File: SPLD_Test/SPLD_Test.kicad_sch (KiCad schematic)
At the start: 34 parts, among them J1 SPI OLED 1.3in, J2 USB_C_Receptacle_PowerOnly_6P, J3 Conn_02x09_Top_Bottom, J4 SWD, J5 Conn_02x09_Top_Bottom, J6 Conn_02x09_Top_Bottom, SW1 SW_MEC_5E, SW2 SW_MEC_5E, SW3 SW_MEC_5E, SW4 SW_MEC_5E, U1 STM32F030K6Tx, U2 EA8105, U3 CA56-12CGKWA, U4 ATF1502ASV-xAx44

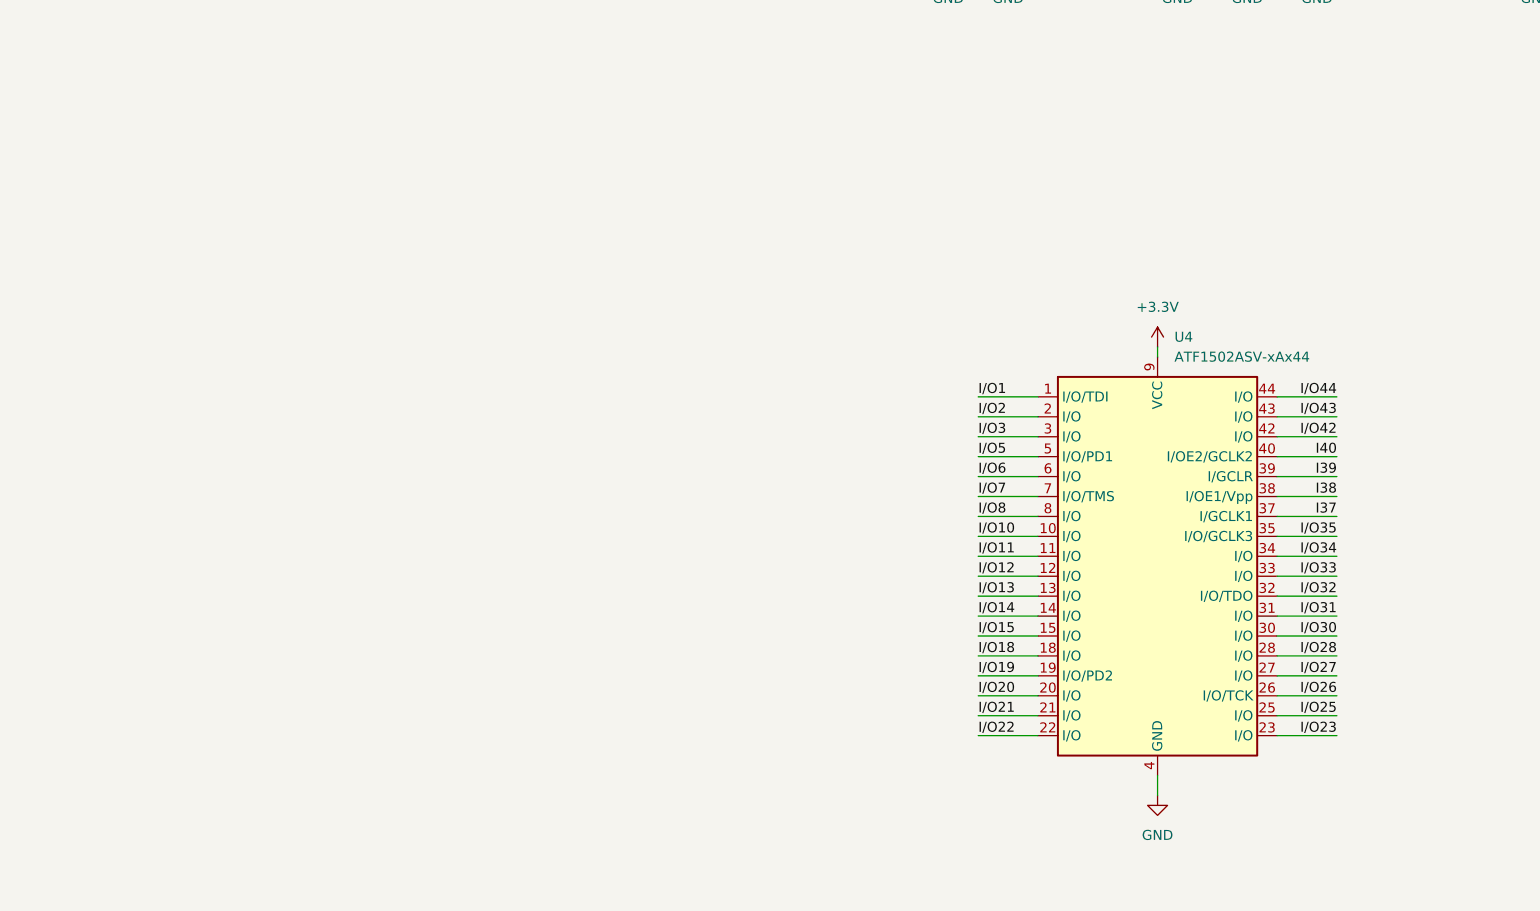
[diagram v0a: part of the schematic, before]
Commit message: progress: CPLD Big Change
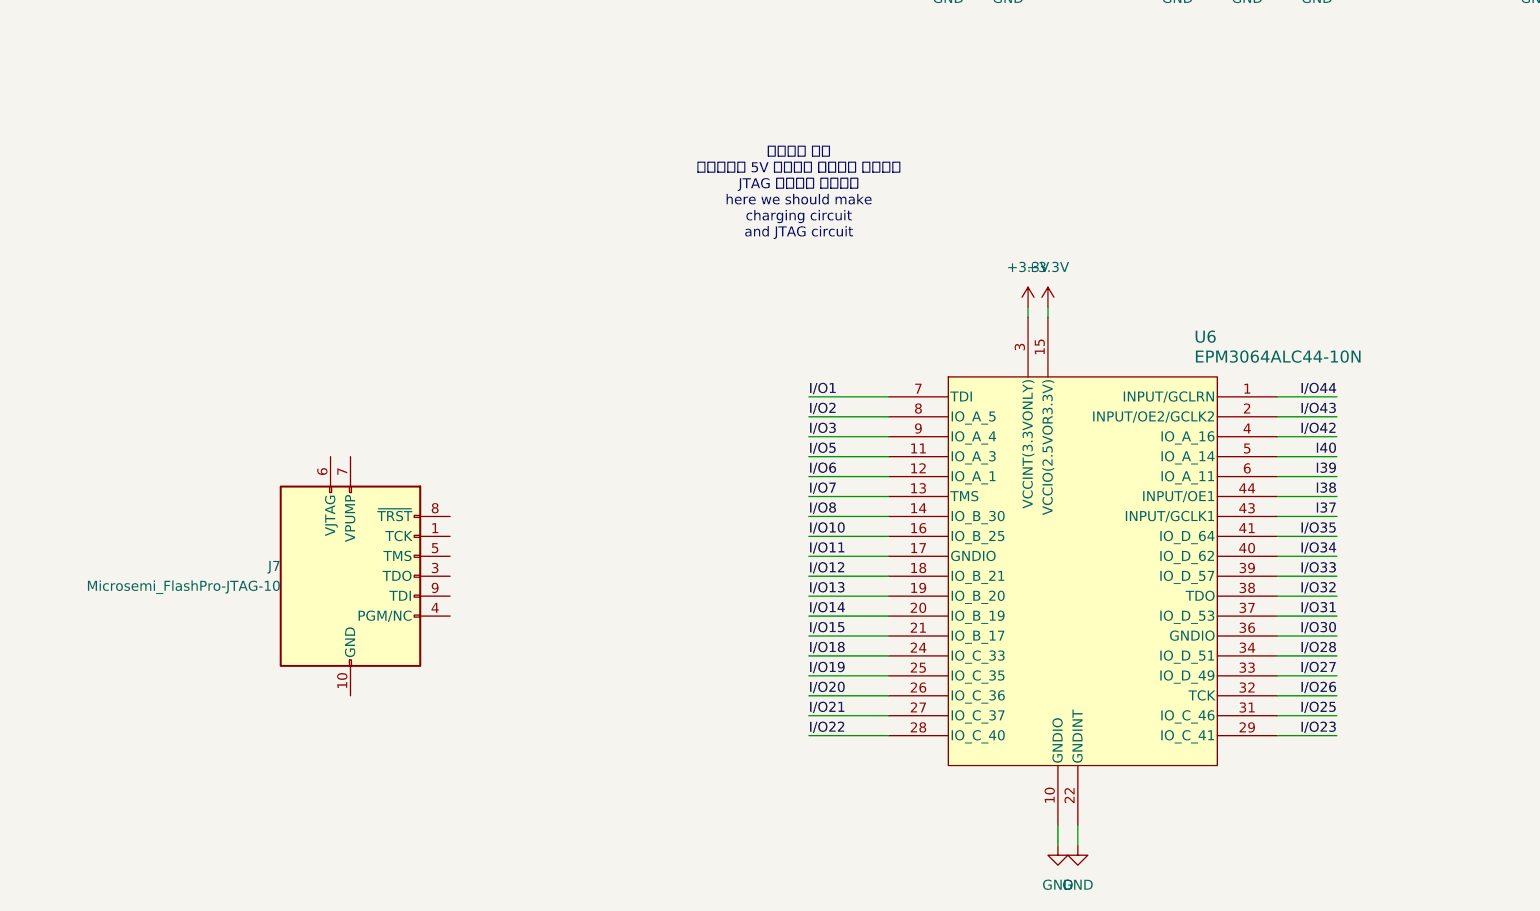
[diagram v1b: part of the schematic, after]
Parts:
- removed U4: ATF1502ASV-xAx44, Package_LCC:PLCC-44_THT-Socket, symbol CPLD_Microchip:ATF1502ASV-xAx44
- added J7: Microsemi_FlashPro-JTAG-10, Connector_IDC:IDC-Header_2x05_P2.54mm_Vertical, symbol Connector:Microsemi_FlashPro-JTAG-10
- added U6: EPM3064ALC44-10N, Package_LCC:PLCC-44_THT-Socket, symbol GH_LIBRARIES:EPM3064ALC44-10N
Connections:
- net +3.3V: now also U6.15 (VCCIO(2.5VOR3.3V)), U6.23 (VCCINT(3.3VONLY)), U6.3 (VCCINT(3.3VONLY)), U6.35 (VCCIO(2.5VOR3.3V))
- net GND: now also U6.10 (GNDIO), U6.22 (GNDINT), U6.30 (GNDIO), U6.42 (GNDINT)
- net I37: now also U6.43 (INPUT/GCLK1)
- net I38: now also U6.44 (INPUT/OE1)
- net I39: now also U6.6 (IO_A_11)
- net I40: now also U6.5 (IO_A_14)
- net I/O1: now also U6.7 (TDI)
- net I/O10: now also U6.16 (IO_B_25)
- net I/O11: now also U6.17 (GNDIO)
- net I/O12: now also U6.18 (IO_B_21)
- net I/O13: now also U6.19 (IO_B_20)
- net I/O14: now also U6.20 (IO_B_19)
- net I/O15: now also U6.21 (IO_B_17)
- net I/O18: now also U6.24 (IO_C_33)
- net I/O19: now also U6.25 (IO_C_35)
- net I/O2: now also U6.8 (IO_A_5)
- net I/O20: now also U6.26 (IO_C_36)
- net I/O21: now also U6.27 (IO_C_37)
- net I/O22: now also U6.28 (IO_C_40)
- net I/O23: now also U6.29 (IO_C_41)
- net I/O25: now also U6.31 (IO_C_46)
- net I/O26: now also U6.32 (TCK)
- net I/O27: now also U6.33 (IO_D_49)
- net I/O28: now also U6.34 (IO_D_51)
- net I/O3: now also U6.9 (IO_A_4)
- net I/O30: now also U6.36 (GNDIO)
- net I/O31: now also U6.37 (IO_D_53)
- net I/O32: now also U6.38 (TDO)
- net I/O33: now also U6.39 (IO_D_57)
- net I/O34: now also U6.40 (IO_D_62)
- net I/O35: now also U6.41 (IO_D_64)
- net I/O42: now also U6.4 (IO_A_16)
- net I/O43: now also U6.2 (INPUT/OE2/GCLK2)
- net I/O44: now also U6.1 (INPUT/GCLRN)
- net I/O5: now also U6.11 (IO_A_3)
- net I/O6: now also U6.12 (IO_A_1)
- net I/O7: now also U6.13 (TMS)
- net I/O8: now also U6.14 (IO_B_30)
- new net: J7.10 (GND), J7.2 (GND)
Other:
- note added: "여기다가 그거 충전회로와 5V 승압회로 만들어서 적용하기 JTAG 만들어서 적용하기 here we should make charging circuit and JTAG circuit"
